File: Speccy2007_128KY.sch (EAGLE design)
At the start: 122 parts, among them J1 0, J2 0, J3 0, X1 5V, X2 SCART-F, X3 PS/2 KB, X3P KB, X4 SD Card, X5 ByteBlaster, X6 AVRISP

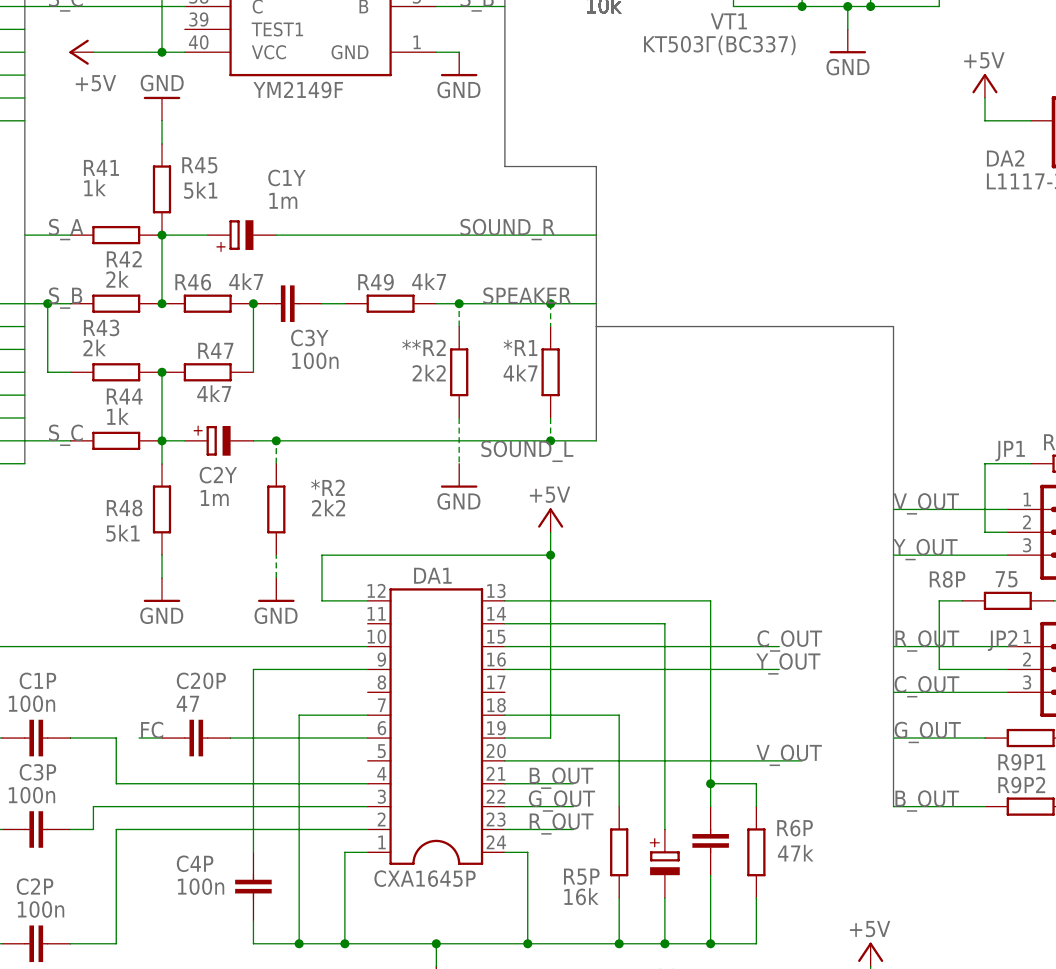
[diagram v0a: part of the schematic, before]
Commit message: clear
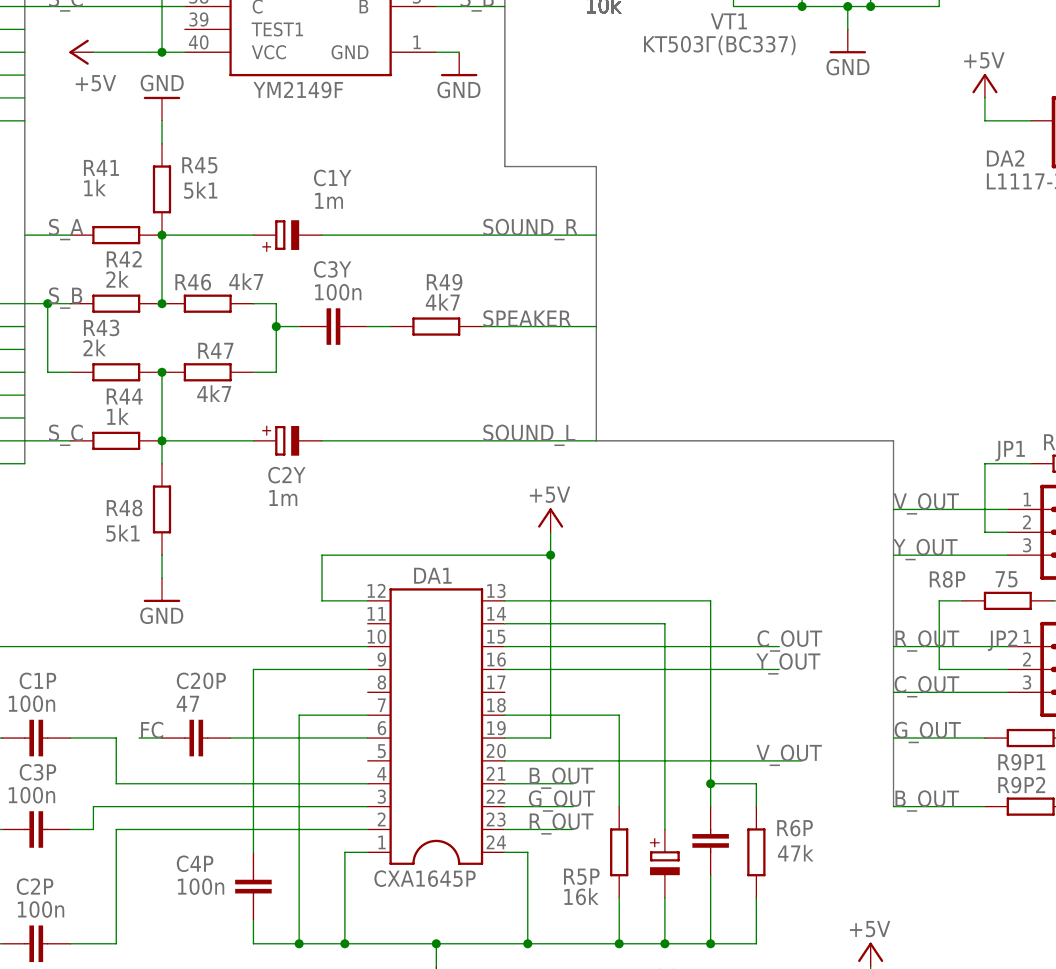
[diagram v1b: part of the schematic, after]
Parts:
- removed **R2: 2k2, rcl:R-EU_R1206
- removed *R1: 4k7, rcl:R-EU_R0805
- removed *R2: 2k2, rcl:R-EU_R0805
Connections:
- net GND: no longer **R2.1, *R2.1
- net SOUND_L: no longer *R1.1, *R2.2
- net SPEAKER: no longer **R2.2, *R1.2
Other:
- moved on the sheet: C1Y, C2Y, C3Y, R49
